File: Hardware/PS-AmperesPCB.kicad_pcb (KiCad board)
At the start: 2 copper layers, 81.4 x 95.2 mm, 160 parts, among them IC1 SN74AHC1G32DBVR, IC2 INA241A4IDR, IC3 AMC1350DWVR, IC4 TLV9002QDRQ1, IC5 LM76202QPWPRQ1, J1 PeripheralCAN, J2 PeripheralCAN, J3 SWD, J4 Conn_01x02_Pin, J5 USB4120-03-C, J6 Scrut Conn, SW1 RST, SW2 BOOT, SW3 Scrut Select, U1 LT1963AEST-3.3#TRPBF, U2 TPS5405DR, U3 TPS2115ADRBR, U4 LT1963AEST-3.3#TRPBF, U5 STM32L431CBTx, U6 TCAN337, U7 CDSOT23-T24CAN, U8 CP2102N-A02-GQFN24, U9 REF35125QDBVR, Y1 8M

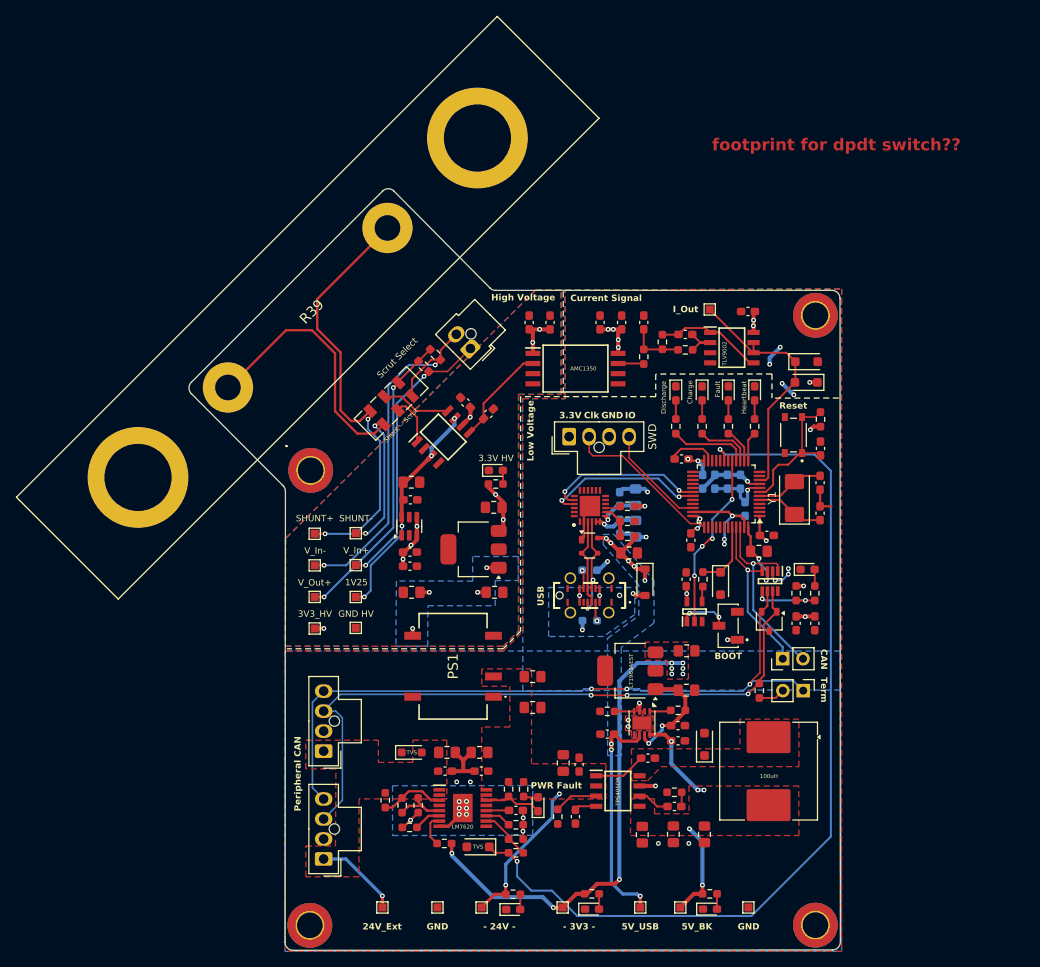
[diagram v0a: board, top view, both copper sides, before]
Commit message: i don't know what I changed
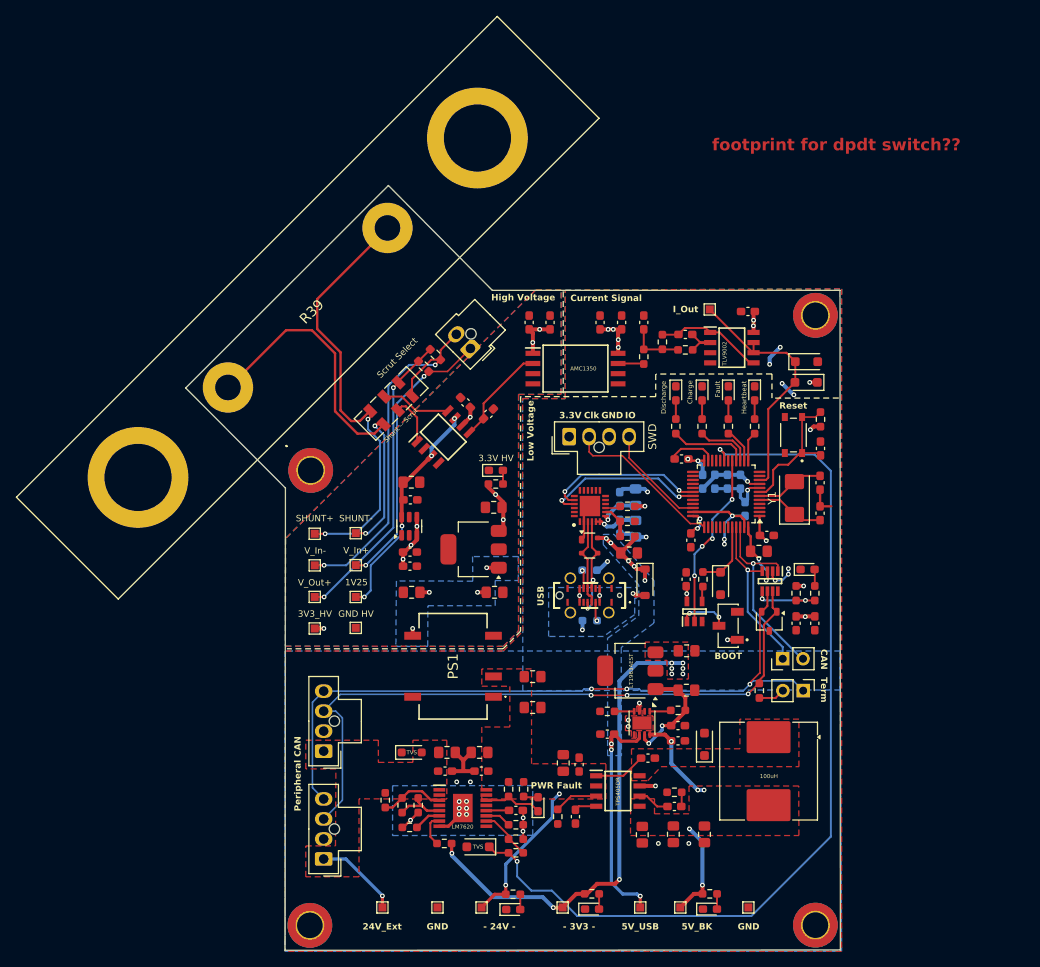
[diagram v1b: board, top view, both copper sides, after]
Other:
- board size 81.4 x 95.2 mm -> 81.8 x 95.6 mm
